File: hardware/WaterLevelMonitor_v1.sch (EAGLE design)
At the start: 49 parts, among them J1 AVR_SPI_PRG_6PTH, J12 D24V5F5, J16 D24V5F5, J17 RJ45, J21 POWER_JACKPTH_BREAD, J6 D24V5F5, Q2 2N3904, Q3 NDP6020P, U1 ATMEGA328P_PDIP

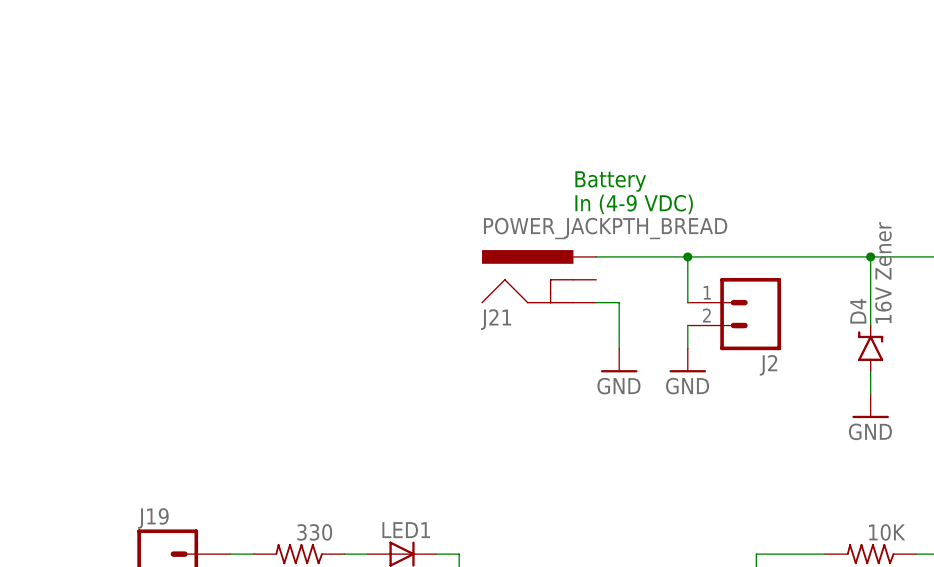
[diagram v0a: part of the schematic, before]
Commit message: Add files via upload
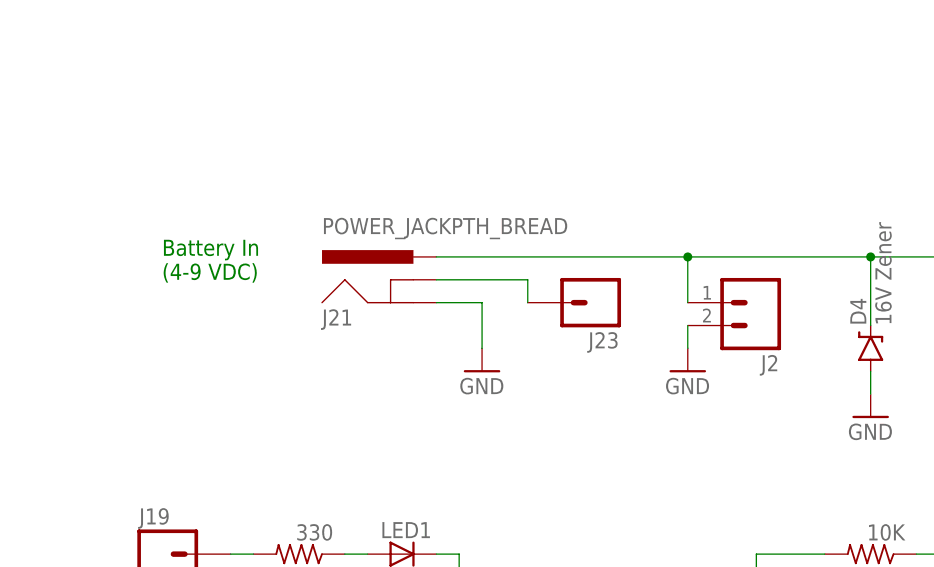
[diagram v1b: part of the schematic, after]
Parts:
- added J23: (no value), SparkFun-Connectors:M01PTH_NO_SILK_YES_STOP
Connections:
- new net N$16: J21.GNDBREAK, J23.1
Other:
- moved on the sheet: J21
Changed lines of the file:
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@@
 <part name="GND11" library="SparkFun-Aesthetics" deviceset="GND" device=""/>
 <part name="J21" library="SparkFun-Connectors" deviceset="POWER_JACK" device="PTH_BREAD"/>
+<part name="J23" library="SparkFun-Connectors" deviceset="M01" device="PTH_NO_SILK_YES_STOP"/>
 </parts>
 <sheets>
 <sheet>
 <plain>
-<text x="-55.88" y="223.52" size="1.778" layer="91">Battery
-In (4-9 VDC)</text>
+<text x="-101.6" y="215.9" size="1.778" layer="91">Battery In
+(4-9 VDC)</text>
 <wire x1="-137.16" y1="144.78" x2="-96.52" y2="144.78" width="0.1524" layer="97" style="longdash"/>
 <wire x1="-96.52" y1="144.78" x2="-96.52" y2="114.3" width="0.1524" layer="97" style="longdash"/>
@@
 <instance part="J13" gate="J$1" x="66.04" y="154.94" rot="R180"/>
 <instance part="GND21" gate="1" x="40.64" y="149.86"/>
-<instance part="GND7" gate="1" x="-50.8" y="205.74"/>
+<instance part="GND7" gate="1" x="-66.04" y="205.74"/>
 <instance part="GND28" gate="1" x="71.12" y="104.14"/>
 <instance part="GND29" gate="1" x="71.12" y="91.44"/>
@@
 <instance part="J2" gate="G$1" x="-35.56" y="213.36" rot="R180"/>
 <instance part="GND11" gate="1" x="-43.18" y="205.74"/>
-<instance part="J21" gate="G$1" x="-55.88" y="210.82"/>
+<instance part="J21" gate="G$1" x="-73.66" y="210.82"/>
+<instance part="J23" gate="G$1" x="-53.34" y="213.36" rot="R180"/>
 </instances>
 <busses>
@@
 <segment>
 <pinref part="GND7" gate="1" pin="GND"/>
-<wire x1="-53.34" y1="213.36" x2="-50.8" y2="213.36" width="0.1524" layer="91"/>
-<wire x1="-50.8" y1="213.36" x2="-50.8" y2="208.28" width="0.1524" layer="91"/>
+<wire x1="-71.12" y1="213.36" x2="-66.04" y2="213.36" width="0.1524" layer="91"/>
+<wire x1="-66.04" y1="213.36" x2="-66.04" y2="208.28" width="0.1524" layer="91"/>
 <pinref part="J21" gate="G$1" pin="GND"/>
 </segment>
@@
 <wire x1="20.32" y1="241.3" x2="25.4" y2="241.3" width="0.1524" layer="91"/>
 <junction x="20.32" y="218.44"/>
-<wire x1="-53.34" y1="218.44" x2="-43.18" y2="218.44" width="0.1524" layer="91"/>
+<wire x1="-71.12" y1="218.44" x2="-43.18" y2="218.44" width="0.1524" layer="91"/>
 <junction x="-22.86" y="218.44"/>
 <pinref part="J2" gate="G$1" pin="1"/>
@@
 </segment>
 </net>
+<net name="N$16" class="0">
+<segment>
+<pinref part="J21" gate="G$1" pin="GNDBREAK"/>
+<pinref part="J23" gate="G$1" pin="1"/>
+<wire x1="-71.12" y1="215.9" x2="-60.96" y2="215.9" width="0.1524" layer="91"/>
+<wire x1="-60.96" y1="215.9" x2="-60.96" y2="213.36" width="0.1524" layer="91"/>
+</segment>
+</net>
